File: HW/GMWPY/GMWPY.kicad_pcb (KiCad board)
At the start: 4 copper layers, 85 x 55 mm, 125 parts, among them J1 USB_A, J2 Conn_02x02_Odd_Even, J3 Conn_01x10, J4 Micro_SD_Card_Det, Q1 Q_PJFET_DSG, SW1 MCU_RESET, SW2 MCU_RESET, U1 AMS1117-3.3, U10 TSV991ILT, U11 TSV991ILT, U12 TSV991ILT, U13 LM4040DBZ-2.0, U14 ESP32-S3-WROOM-1, U2 SRV05-4, U3 USEQGCDACH4100, U4 TSV991ILT, U5 MCP3422, U6 TSV991ILT, U7 BME280, U8 MCP3422, U9 EC4-1000-H2

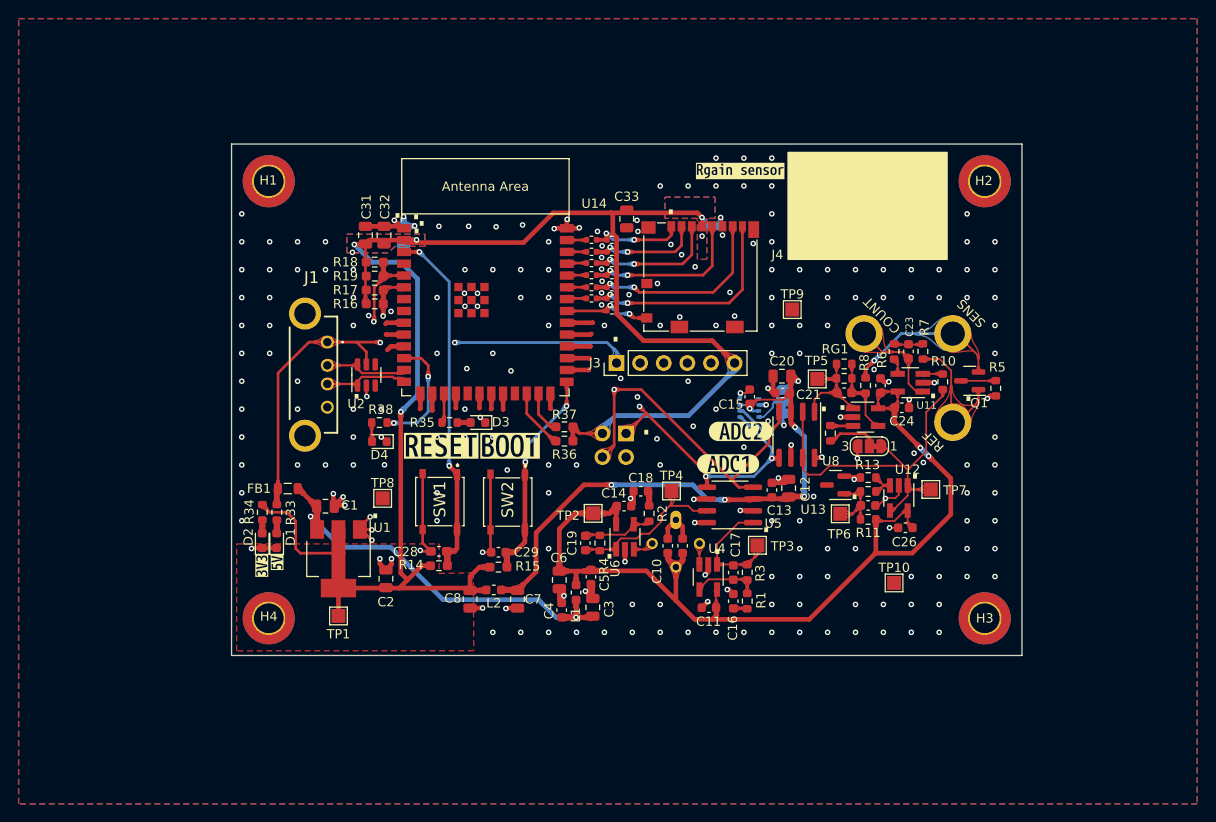
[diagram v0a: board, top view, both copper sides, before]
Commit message: b
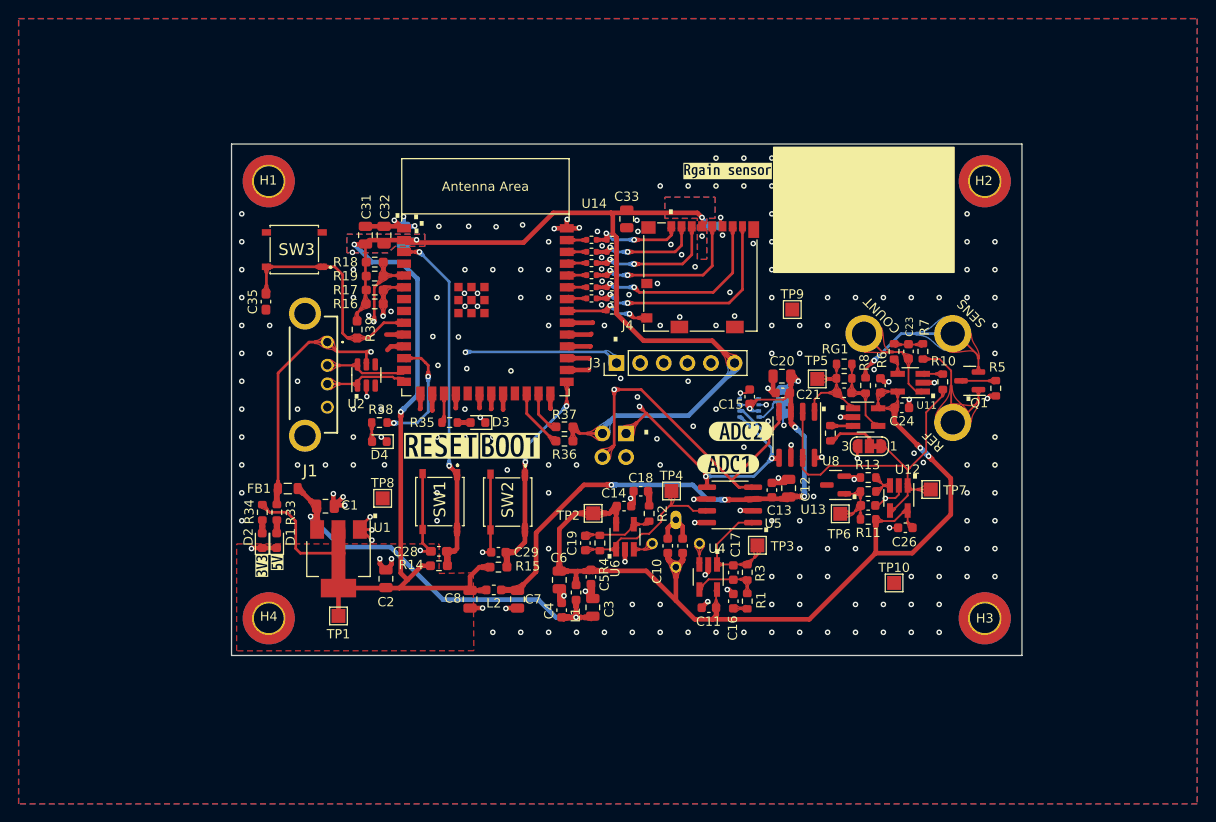
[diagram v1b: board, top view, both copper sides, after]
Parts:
- added C35: 100n, Capacitor_SMD:C_0603_1608Metric_Pad1.08x0.95mm_HandSolder, F.Cu at (53.7, 67.0)
- added R39: 10k, Resistor_SMD:R_0603_1608Metric_Pad0.98x0.95mm_HandSolder, F.Cu at (63.5, 70.0)
- added SW3: MCU_RESET, SamacSys_Parts:PTS526SK15SMTR2LFS, F.Cu at (56.8, 61.4)
- moved kibuzzard-640733B2 1.35 mm to (103.3, 52.9)
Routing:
- net GPIO_16: track 2.05 -> 25.3 mm
- net +3V3: track 187.0 -> 189.3 mm
- net VBUS: track 56.4 -> 54.3 mm
- net GND: vias 261 -> 254
